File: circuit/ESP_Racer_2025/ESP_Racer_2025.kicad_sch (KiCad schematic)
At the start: 19 parts, among them IC1 XCL102D333CR-G, J1 Conn_LED_1, J2 Conn_LED_2, J3 Conn_Servo, U1 DRV8835DSST, U2 SFV12R-2STE1LF, U3 ESP32-C3-WROOM-02

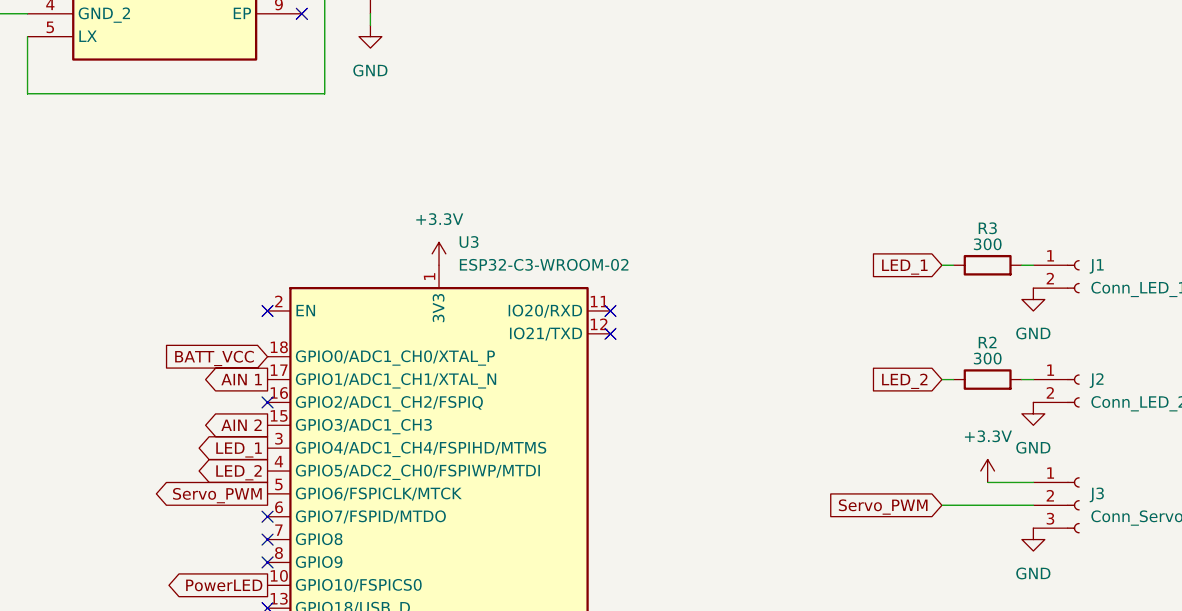
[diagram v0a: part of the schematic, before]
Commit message: update firmware
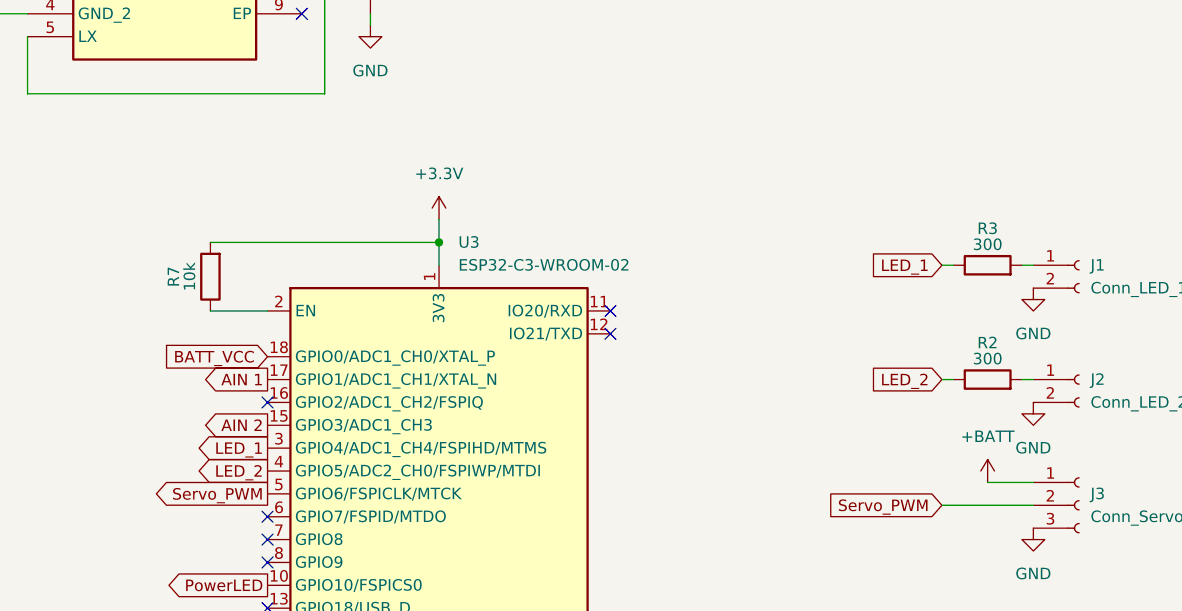
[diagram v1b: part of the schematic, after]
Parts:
- added R7: 10k, Resistor_SMD:R_0603_1608Metric_Pad0.98x0.95mm_HandSolder, symbol Device:R
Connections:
- net +3.3V: now also R7.2; no longer J3.1 (Pin_1)
- net +BATT: now also J3.1 (Pin_1)
- net at U3.2 (EN): now also R7.1
- no-connect marks 10 -> 9
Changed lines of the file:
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@@
 	)
 	(junction
+		(at 184.15 76.2)
+		(diameter 0)
+		(color 0 0 0 0)
+	)
+	(junction
 		(at 93.98 80.01)
 		(diameter 0)
@@
 	)
 	(no_connect
-		(at 165.1 83.82)
-	)
-	(no_connect
 		(at 165.1 109.22)
 	)
@@
 	(wire
 		(pts
+			(xy 184.15 76.2) (xy 184.15 78.74)
+		)
+		(stroke
+			(width 0)
+			(type default)
+		)
+	)
+	(wire
+		(pts
 			(xy 120.65 137.16) (xy 120.65 140.97)
 		)
@@
 	(wire
 		(pts
+			(xy 184.15 73.66) (xy 184.15 76.2)
+		)
+		(stroke
+			(width 0)
+			(type default)
+		)
+	)
+	(wire
+		(pts
 			(xy 153.67 31.75) (xy 171.45 31.75)
 		)
@@
 	(wire
 		(pts
+			(xy 158.75 76.2) (xy 184.15 76.2)
+		)
+		(stroke
+			(width 0)
+			(type default)
+		)
+	)
+	(wire
+		(pts
 			(xy 96.52 82.55) (xy 96.52 87.63)
 		)
@@
 	(wire
 		(pts
+			(xy 158.75 83.82) (xy 165.1 83.82)
+		)
+		(stroke
+			(width 0)
+			(type default)
+		)
+	)
+	(wire
+		(pts
 			(xy 121.92 31.75) (xy 121.92 34.29)
 		)
@@
 	)
 	(symbol
+		(lib_id "Device:R")
+		(at 158.75 80.01 180)
+		(unit 1)
+		(exclude_from_sim no)
+		(in_bom yes)
+		(on_board yes)
+		(dnp no)
+		(property "Reference" "R7"
+			(at 154.686 80.01 90)
+			(effects
+				(font
+					(size 1.27 1.27)
+				)
+			)
+		)
+		(property "Value" "10k"
+			(at 156.464 80.01 90)
+			(effects
+				(font
+					(size 1.27 1.27)
+				)
+			)
+		)
+		(property "Footprint" "Resistor_SMD:R_0603_1608Metric_Pad0.98x0.95mm_HandSolder"
+			(at 160.528 80.01 90)
+			(effects
+				(font
+					(size 1.27 1.27)
+				)
+				(hide yes)
+			)
+		)
+		(property "Datasheet" "~"
+			(at 158.75 80.01 0)
+			(effects
+				(font
+					(size 1.27 1.27)
+				)
+				(hide yes)
+			)
+		)
+		(property "Description" "Resistor"
+			(at 158.75 80.01 0)
+			(effects
+				(font
+					(size 1.27 1.27)
+				)
+				(hide yes)
+			)
+		)
+		(pin "1"
+		)
+		(pin "2"
+		)
+		(instances
+			(project "ESP_Racer_2025"
+				(path "/5c50a387-df5f-414d-8825-9a6969b82251"
+					(reference "R7")
+					(unit 1)
+				)
+			)
+		)
+	)
+	(symbol
 		(lib_id "Device:C")
 		(at 130.81 38.1 0)
@@
 	)
 	(symbol
+		(lib_id "power:+BATT")
+		(at 245.11 102.87 0)
+		(unit 1)
+		(exclude_from_sim no)
+		(in_bom yes)
+		(on_board yes)
+		(dnp no)
+		(fields_autoplaced yes)
+		(property "Reference" "#PWR020"
+			(at 245.11 106.68 0)
+			(effects
+				(font
+					(size 1.27 1.27)
+				)
+				(hide yes)
+			)
+		)
+		(property "Value" "+BATT"
+			(at 245.11 97.79 0)
+			(effects
+				(font
+					(size 1.27 1.27)
+				)
+			)
+		)
+		(property "Footprint" ""
+			(at 245.11 102.87 0)
+			(effects
+				(font
+					(size 1.27 1.27)
+				)
+				(hide yes)
+			)
+		)
+		(property "Datasheet" ""
+			(at 245.11 102.87 0)
+			(effects
+				(font
+					(size 1.27 1.27)
+				)
+				(hide yes)
+			)
+		)
+		(property "Description" "Power symbol creates a global label with name \"+BATT\""
+			(at 245.11 102.87 0)
+			(effects
+				(font
+					(size 1.27 1.27)
+				)
+				(hide yes)
+			)
+		)
+		(pin "1"
+		)
+		(instances
+			(project "ESP_Racer_2025"
+				(path "/5c50a387-df5f-414d-8825-9a6969b82251"
+					(reference "#PWR020")
+					(unit 1)
+				)
+			)
+		)
+	)
+	(symbol
 		(lib_id "Connector:Conn_01x02_Socket")
 		(at 255.27 78.74 0)
@@
 	)
 	(symbol
-		(lib_id "power:+3.3V")
-		(at 245.11 102.87 0)
-		(unit 1)
-		(exclude_from_sim no)
-		(in_bom yes)
-		(on_board yes)
-		(dnp no)
-		(fields_autoplaced yes)
-		(property "Reference" "#PWR020"
-			(at 245.11 106.68 0)
-			(effects
-				(font
-					(size 1.27 1.27)
-				)
-				(hide yes)
-			)
-		)
-		(property "Value" "+3.3V"
-			(at 245.11 97.79 0)
-			(effects
-				(font
-					(size 1.27 1.27)
-				)
-			)
-		)
-		(property "Footprint" ""
-			(at 245.11 102.87 0)
-			(effects
-				(font
-					(size 1.27 1.27)
-				)
-				(hide yes)
-			)
-		)
-		(property "Datasheet" ""
-			(at 245.11 102.87 0)
-			(effects
-				(font
-					(size 1.27 1.27)
-				)
-				(hide yes)
-			)
-		)
-		(property "Description" "Power symbol creates a global label with name \"+3.3V\""
-			(at 245.11 102.87 0)
-			(effects
-				(font
-					(size 1.27 1.27)
-				)
-				(hide yes)
-			)
-		)
-		(pin "1"
-		)
-		(instances
-			(project "ESP_Racer_2025"
-				(path "/5c50a387-df5f-414d-8825-9a6969b82251"
-					(reference "#PWR020")
-					(unit 1)
-				)
-			)
-		)
-	)
-	(symbol
 		(lib_id "Device:C")
 		(at 124.46 78.74 0)
@@
 	(symbol
 		(lib_id "power:+3.3V")
-		(at 184.15 78.74 0)
+		(at 184.15 73.66 0)
 		(unit 1)
 		(exclude_from_sim no)
@@
 		(fields_autoplaced yes)
 		(property "Reference" "#PWR015"
-			(at 184.15 82.55 0)
+			(at 184.15 77.47 0)
 			(effects
 				(font
@@
 		)
 		(property "Value" "+3.3V"
-			(at 184.15 73.66 0)
+			(at 184.15 68.58 0)
 			(effects
 				(font
@@
 		)
 		(property "Footprint" ""
-			(at 184.15 78.74 0)
+			(at 184.15 73.66 0)
 			(effects
 				(font
@@
 		)
 		(property "Datasheet" ""
-			(at 184.15 78.74 0)
+			(at 184.15 73.66 0)
 			(effects
 				(font
@@
 		)
 		(property "Description" "Power symbol creates a global label with name \"+3.3V\""
-			(at 184.15 78.74 0)
+			(at 184.15 73.66 0)
 			(effects
 				(font
